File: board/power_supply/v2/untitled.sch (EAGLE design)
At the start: 20 parts, among them IC1 317EMP, Q1 FDD4141TO252

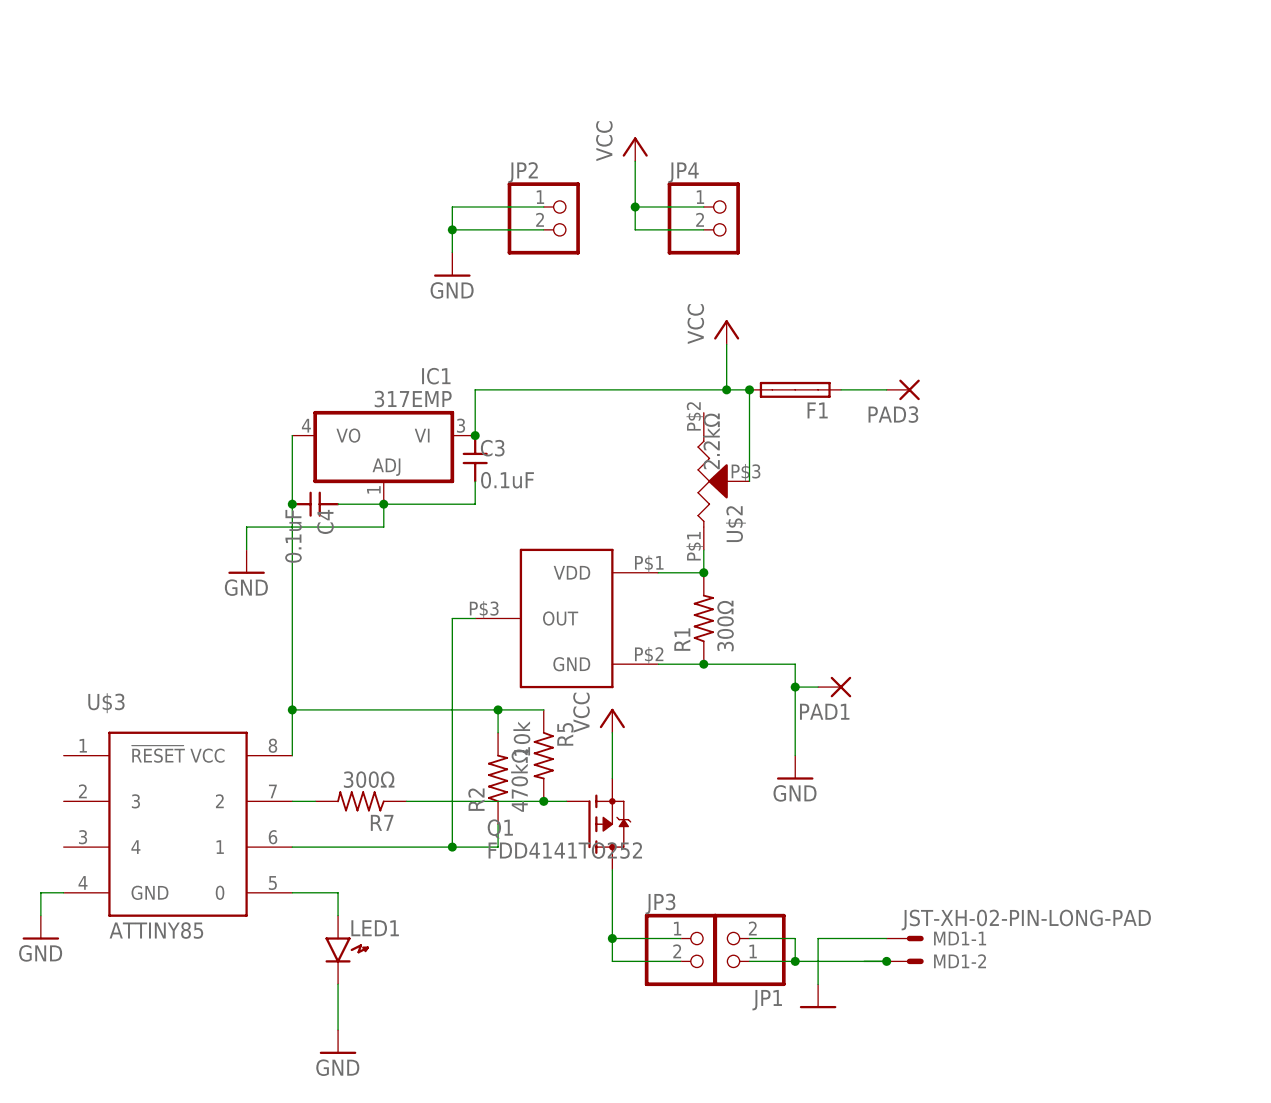
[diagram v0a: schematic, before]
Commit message: marge前のファイル
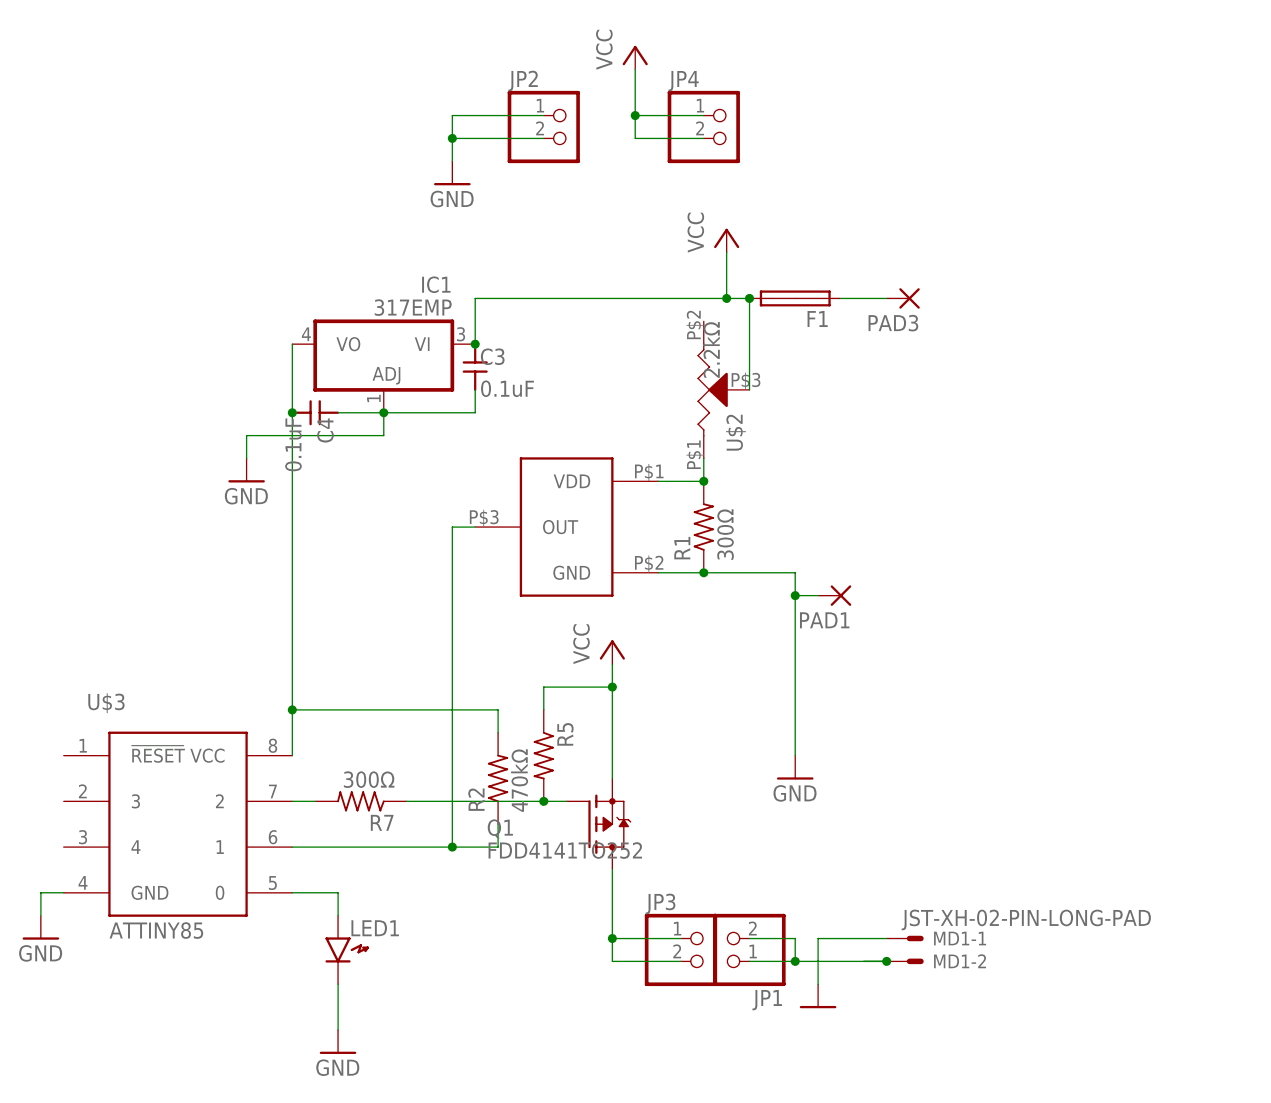
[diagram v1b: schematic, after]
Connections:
- net N$11: no longer R5.1
- net VCC: now also R5.1
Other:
- moved on the sheet: C3, C4, F1, IC1, JP2, JP4, PAD1, PAD3, R1, U$2

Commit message: Revert "Merge remote-tracking branch 'origin/Develop' into feature_#37"
This reverts commit cb103155361e8766478c6830db153463370c0739, reversing
changes made to 84e093fe944e1f8653a6822ff34e6f8740617cb5.
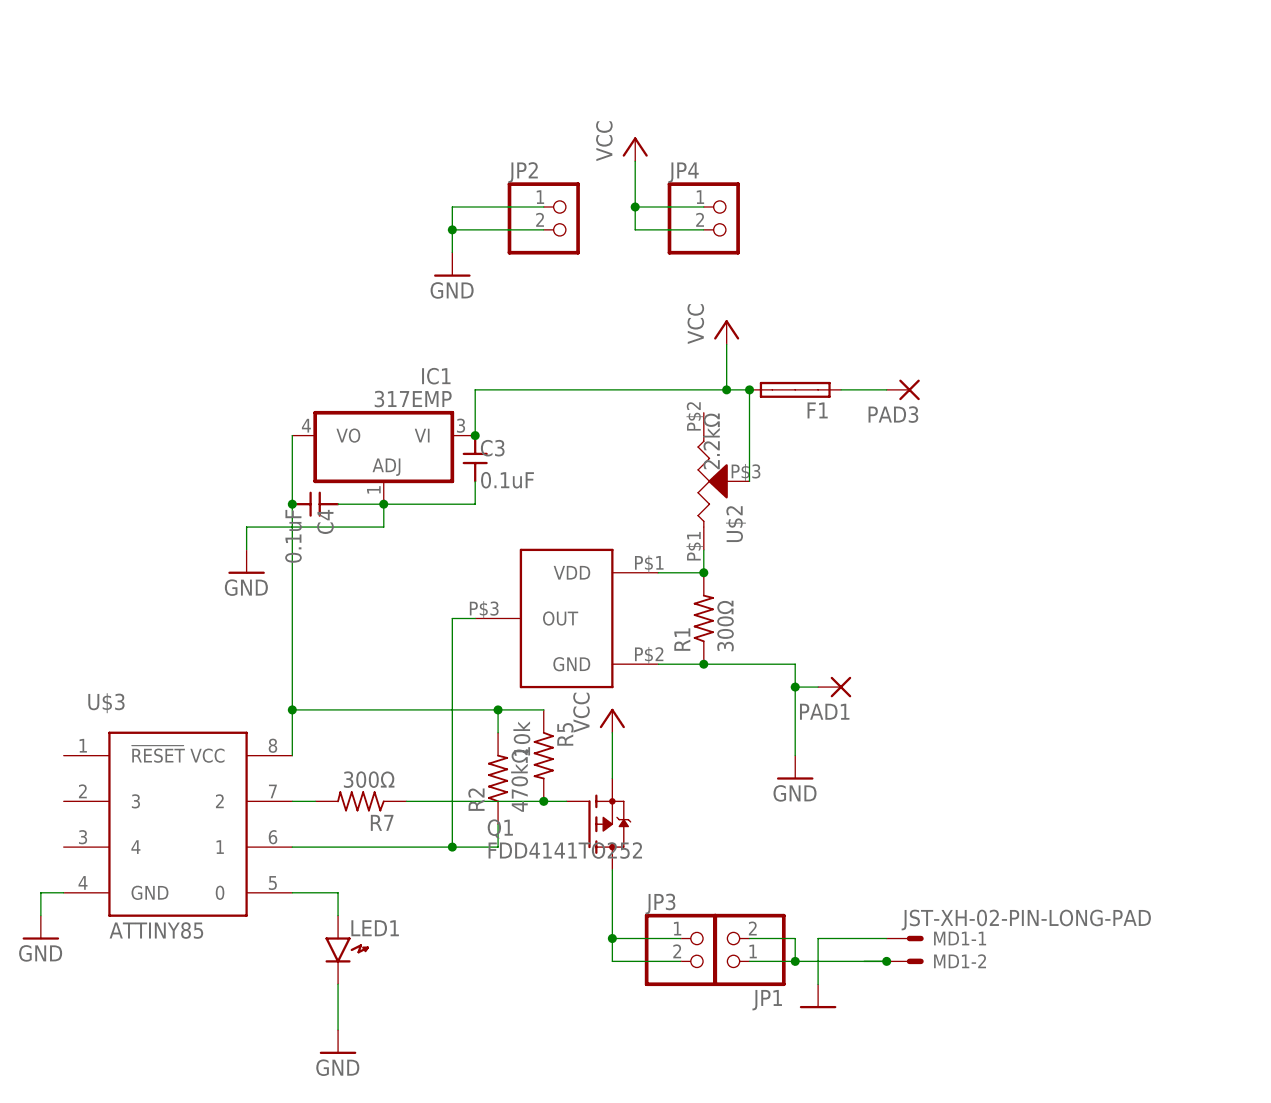
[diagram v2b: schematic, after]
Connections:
- net N$11: now also R5.1
- net VCC: no longer R5.1
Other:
- moved on the sheet: C3, C4, F1, IC1, JP2, JP4, PAD1, PAD3, R1, U$2
